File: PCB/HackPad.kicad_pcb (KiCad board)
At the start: 2 copper layers, 79.2 x 47.2 mm, 10 parts, among them SW1 RotaryEncoder_Switch, SW2 RotaryEncoder_Switch, SW4 SW_Push, SW5 SW_Push, SW6 SW_Push, SW7 SW_Push, U1 Seeed Studio XIAO SAMD21, U2 PCF8574A

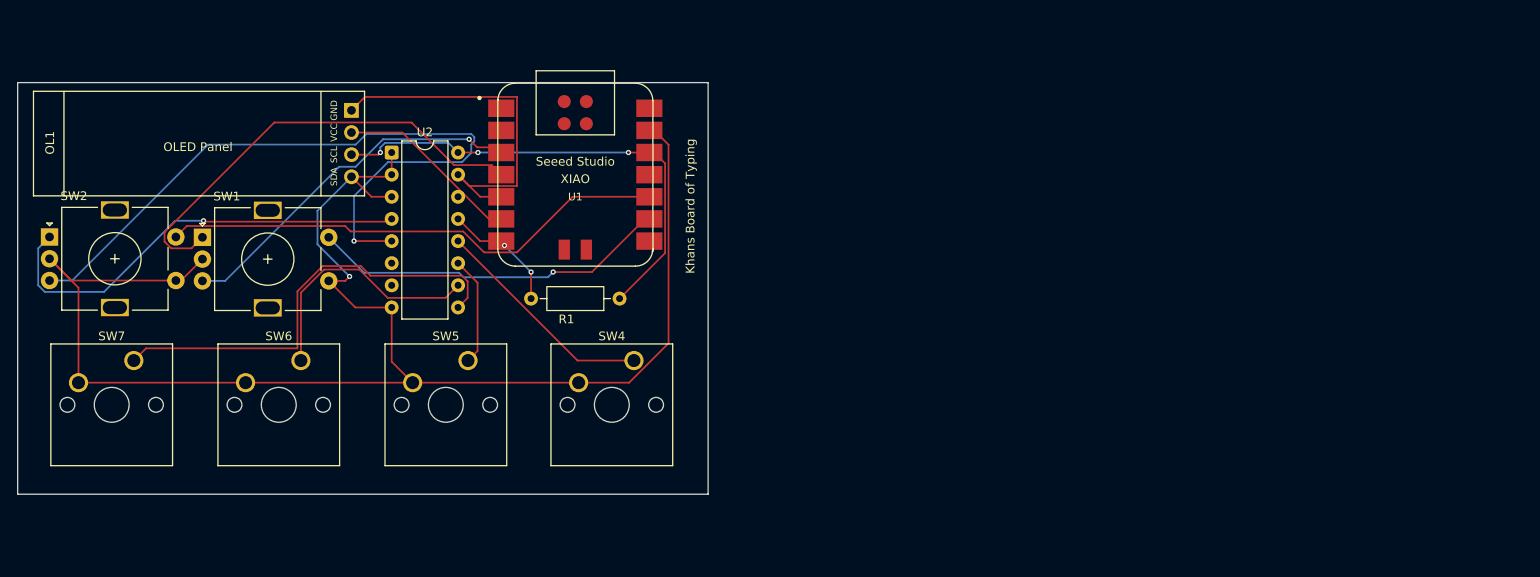
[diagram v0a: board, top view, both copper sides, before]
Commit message: Add files via upload
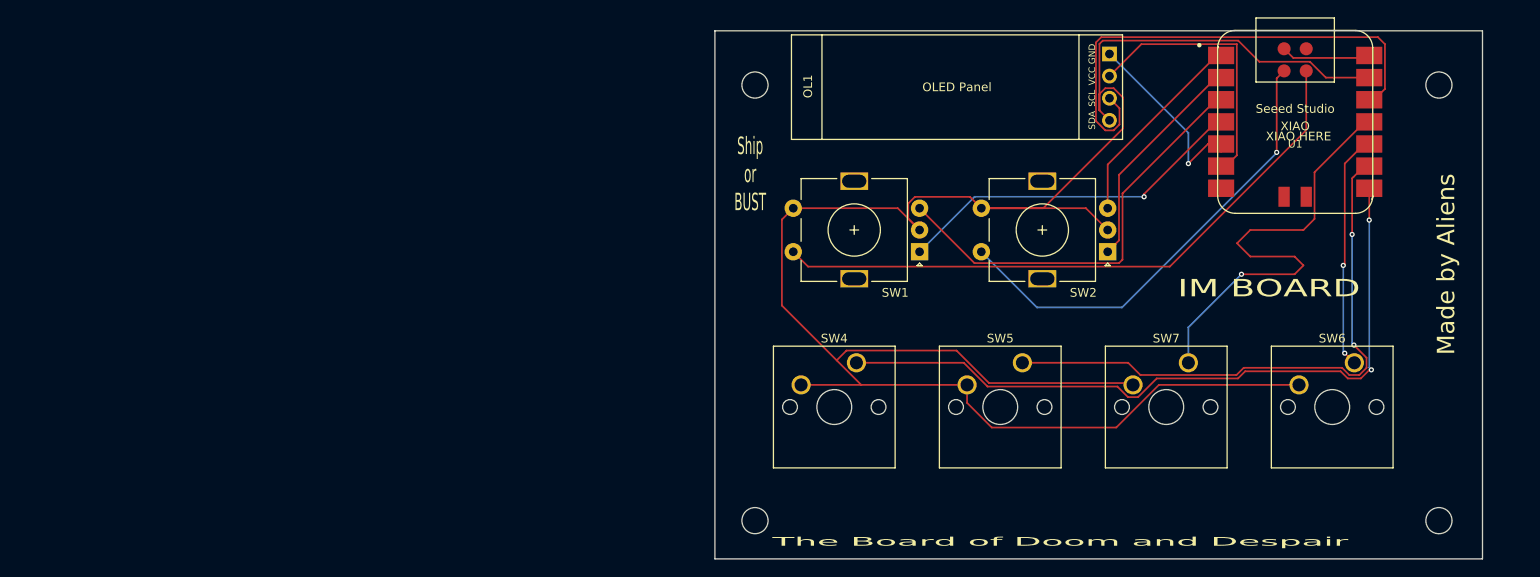
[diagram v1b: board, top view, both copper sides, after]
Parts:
- removed R1: 10k, Resistor_THT:R_Axial_DIN0207_L6.3mm_D2.5mm_P10.16mm_Horizontal
- removed U2: PCF8574A, Package_DIP:DIP-16_W7.62mm
- moved SW2 121.5 mm to (196.5, 106.6), turned to 180 degrees
- moved SW7 121.0 mm to (205.7, 119.4)
- moved SW6 120.9 mm to (224.8, 119.4)
- moved OL1 87.2 mm to (160.2, 81.7)
- moved U1 82.8 mm to (218.0, 91.7)
- moved SW1 82.3 mm to (174.9, 106.6), turned to 180 degrees
- moved SW5 63.6 mm to (186.7, 119.4)
- moved SW4 25.5 mm to (167.6, 119.4)
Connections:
- net VCC renamed Net-(OL1-VCC)
- SW1 pad S2: Net-(U1-PA7_A8_D8_SCK) -> unconnected-(SW1-PadS2)
- SW2 pad A: Net-(U2-P0) -> unconnected-(SW2-PadA)
- SW2 pad B: Net-(U2-P1) -> unconnected-(SW2-PadB)
- SW2 pad S2: Net-(U1-PA5_A9_D9_MISO) -> unconnected-(SW2-PadS2)
- SW4 pad 1: Net-(U2-P7) -> unconnected-(SW4-Pad1)
- SW5 pad 1: Net-(U2-P6) -> Net-(U1-PA7_A8_D8_SCK)
- SW6 pad 1: Net-(U2-P5) -> Net-(U1-PA5_A9_D9_MISO)
- SW7 pad 1: Net-(U2-P4) -> unconnected-(SW7-Pad1)
- U1 pad 1: unconnected-(U1-PA02_A0_D0-Pad1) -> unconnected-(SW2-PadB)
- U1 pad 11: unconnected-(U1-PA6_A10_D10_MOSI-Pad11) -> unconnected-(SW7-Pad1)
- U1 pad 14: unconnected-(U1-5V-Pad14) -> +5V
- U1 pad 15: unconnected-(U1-5V-Pad15) -> +5V
- U1 pad 17: unconnected-(U1-PA31_SWDIO-Pad17) -> unconnected-(SW2-PadS2)
- U1 pad 18: unconnected-(U1-PA30_SWCLK-Pad18) -> unconnected-(SW1-PadS2)
- U1 pad 2: unconnected-(U1-PA4_A1_D1-Pad2) -> unconnected-(SW2-PadA)
- U1 pad 8: unconnected-(U1-PB09_A7_D7_RX-Pad8) -> unconnected-(SW4-Pad1)
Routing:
- net unconnected-(SW4-Pad1): track 0.00 -> 83.7 mm, vias 0 -> 2
- net Net-(U2-P1): track 82.8 -> 0.00 mm, vias 1 -> 0
- net unconnected-(SW1-PadS2): track 0.00 -> 72.9 mm
- net GND: track 178.6 -> 238.0 mm, vias 1 -> 0
- net unconnected-(SW2-PadS2): track 0.00 -> 53.6 mm, vias 0 -> 1
- net unconnected-(SW7-Pad1): track 0.00 -> 53.0 mm, vias 0 -> 1
- net Net-(U2-P4): track 50.8 -> 0.00 mm
- net Net-(U2-P0): track 50.5 -> 0.00 mm, vias 1 -> 0
- net Net-(U1-PA5_A9_D9_MISO): track 58.8 -> 27.2 mm, vias 0 -> 2
- net Net-(U2-P5): track 28.9 -> 0.00 mm
- net Net-(U2-P7): track 25.9 -> 0.00 mm
- net unconnected-(SW2-PadA): track 0.00 -> 25.7 mm
- net Net-(U1-PA7_A8_D8_SCK): track 41.5 -> 66.1 mm, vias 1 -> 2
- net unconnected-(SW2-PadB): track 0.00 -> 23.2 mm
- net Net-(OL1-SDA): track 43.2 -> 22.0 mm, vias 0 -> 1
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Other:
- board size 79.2 x 47.2 mm -> 88.1 x 60.6 mm
- board text added: "IM BOARD"
- board text added: "Made by Aliens"
- board text added: "Ship or BUST"
- board text added: "The Board of Doom and Despair"
- board text added: "XIAO HERE"
- board text removed: "Khans Board of Typing"
